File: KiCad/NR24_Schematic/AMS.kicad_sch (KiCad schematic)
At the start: 4 parts

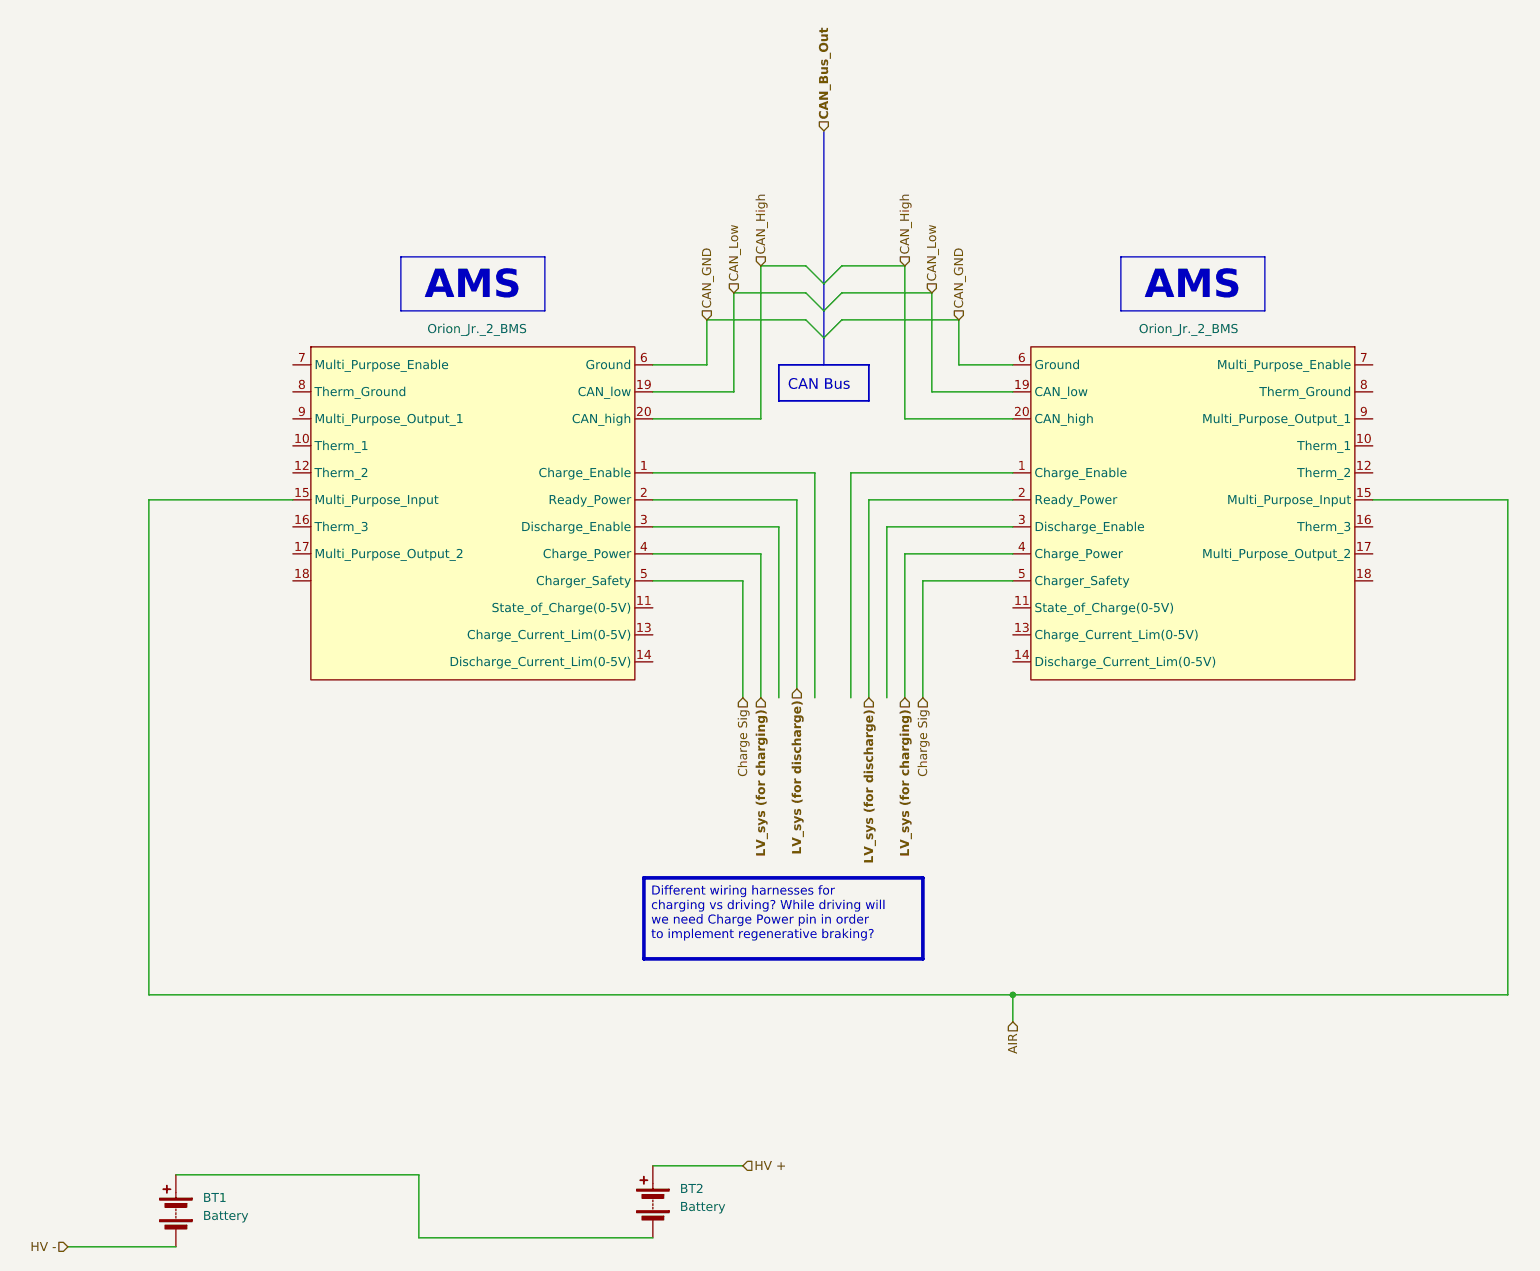
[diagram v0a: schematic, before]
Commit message: Revert "Merge branch 'main' of https://github.com/m241056/NR24"
This reverts commit a926c37884718e9edd96f05865339fc9d3eea559, reversing
changes made to 06e9f39ae517f67b8f5dca544fb6abab47fbdf72.
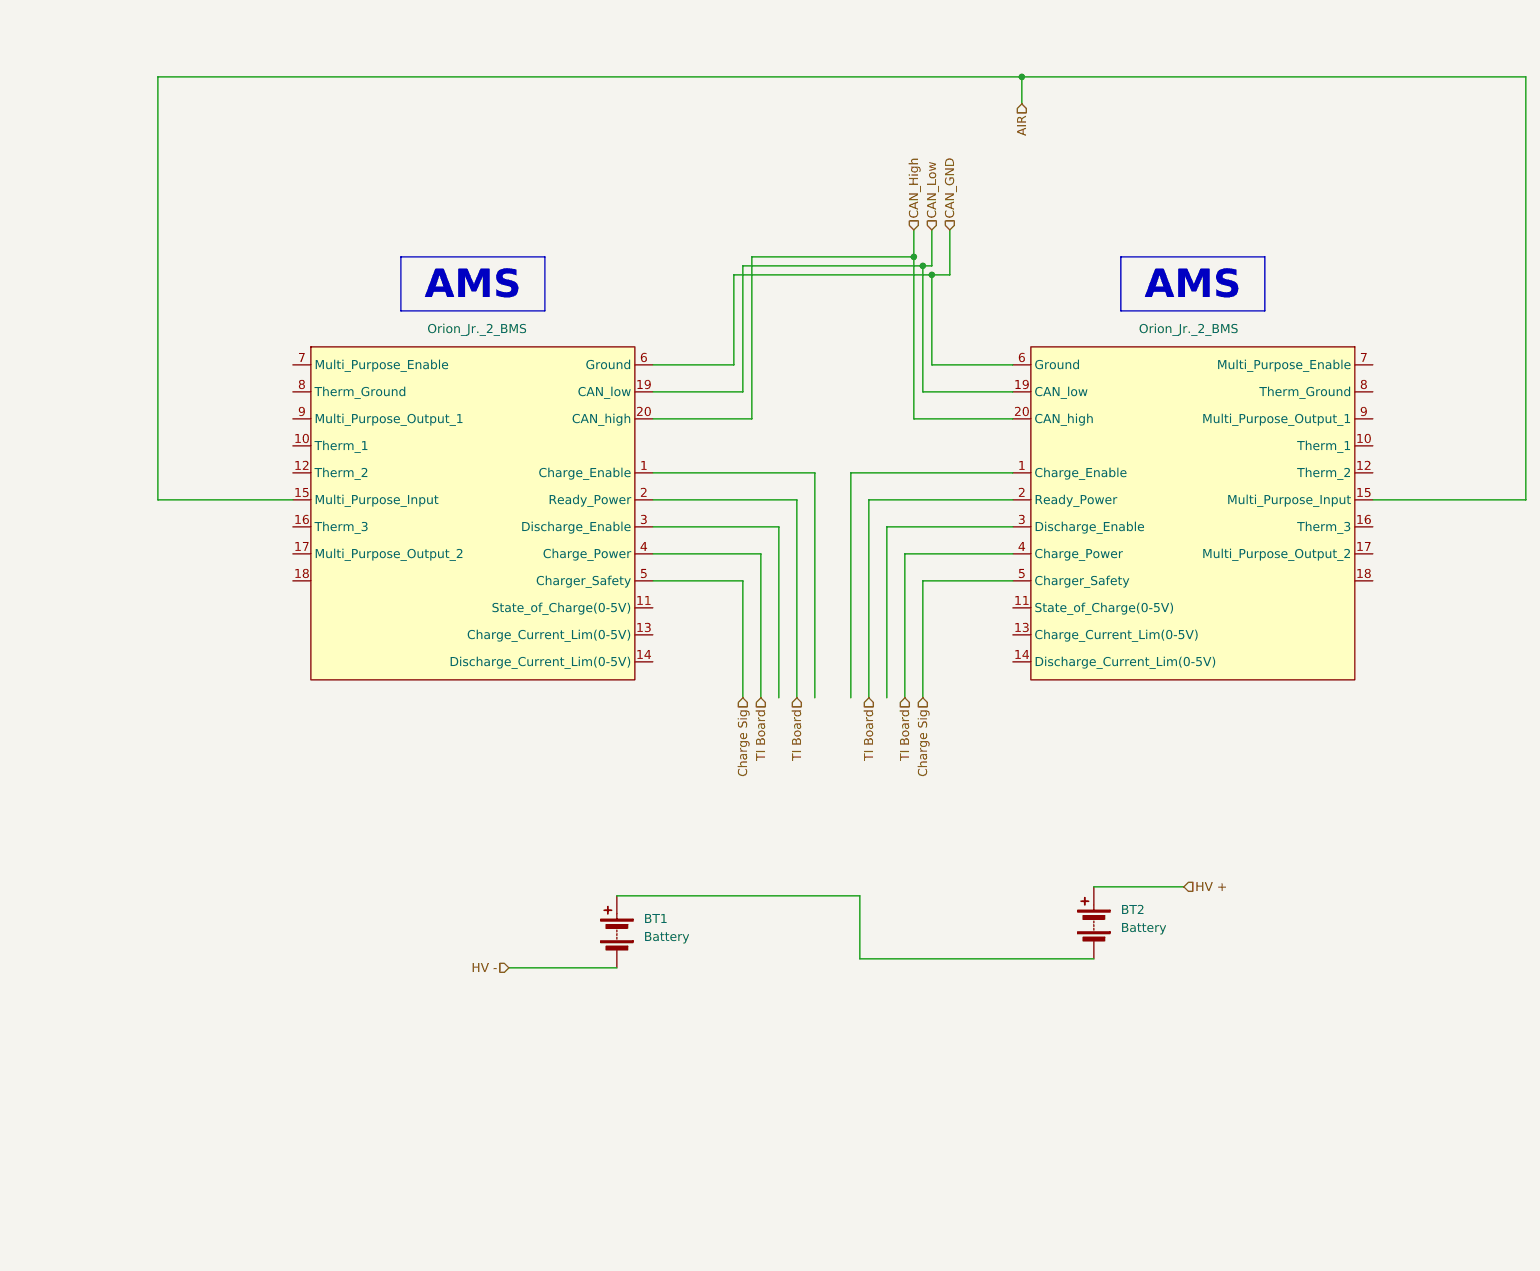
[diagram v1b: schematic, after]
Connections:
- net LV_sys (for discharge) is gone; now on net TI Board: U?.2 (Ready_Power), U?.2 (Ready_Power)
- net LV_sys (for charging) renamed TI Board
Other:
- note removed: "CAN Bus"
- moved on the sheet: BT1, BT2
